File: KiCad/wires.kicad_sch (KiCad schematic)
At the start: 3 parts, among them U1 LT1762

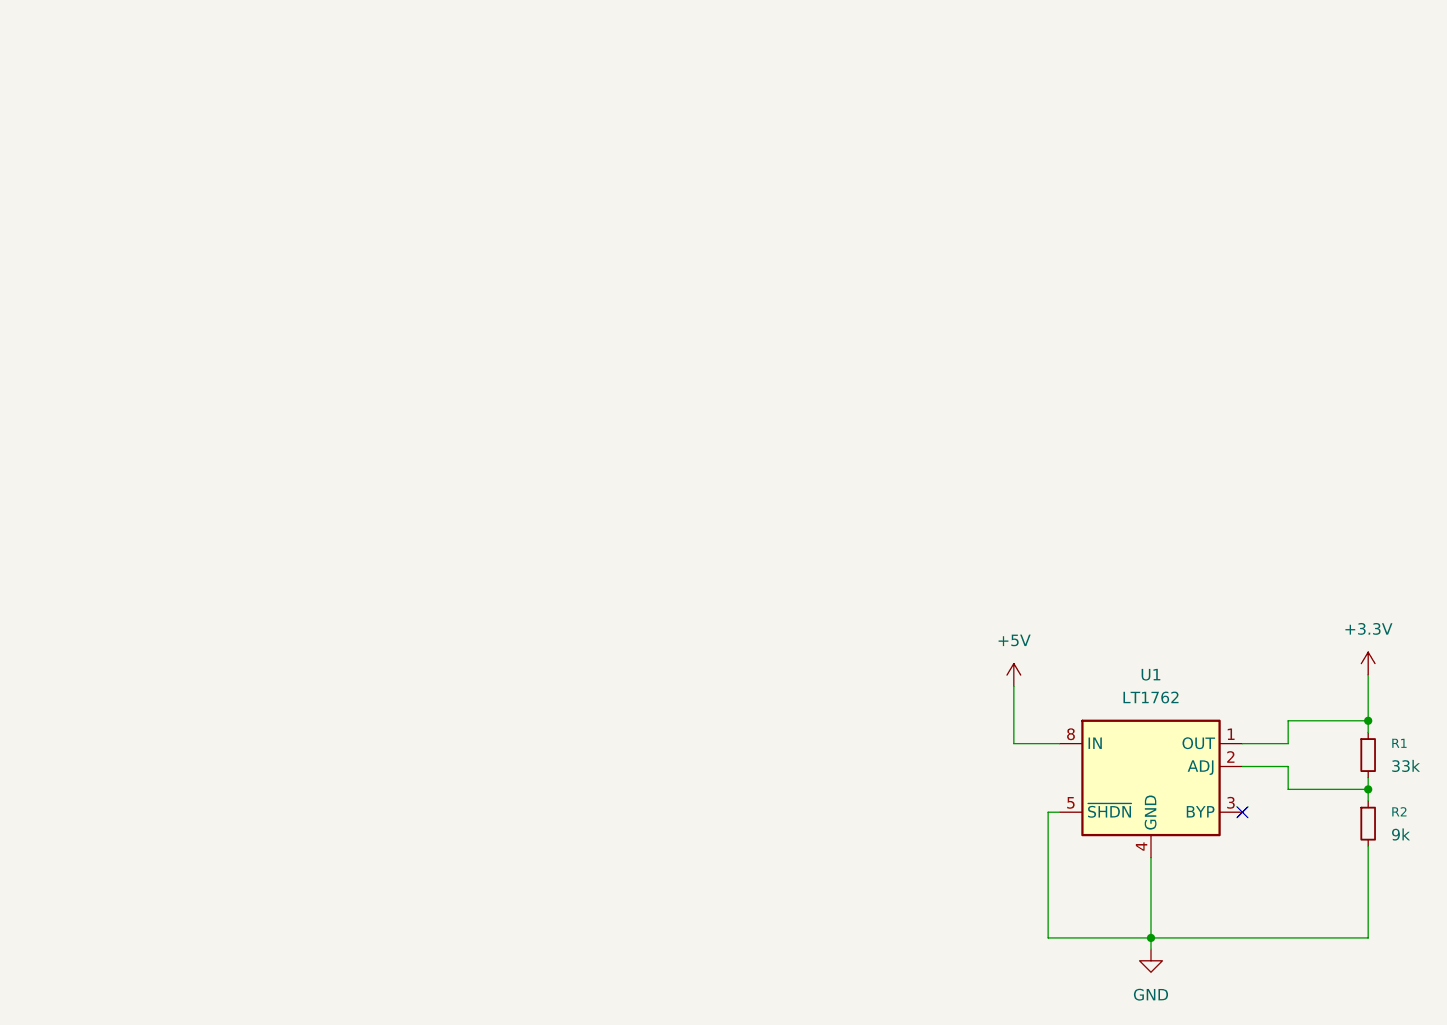
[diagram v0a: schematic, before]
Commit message: Update
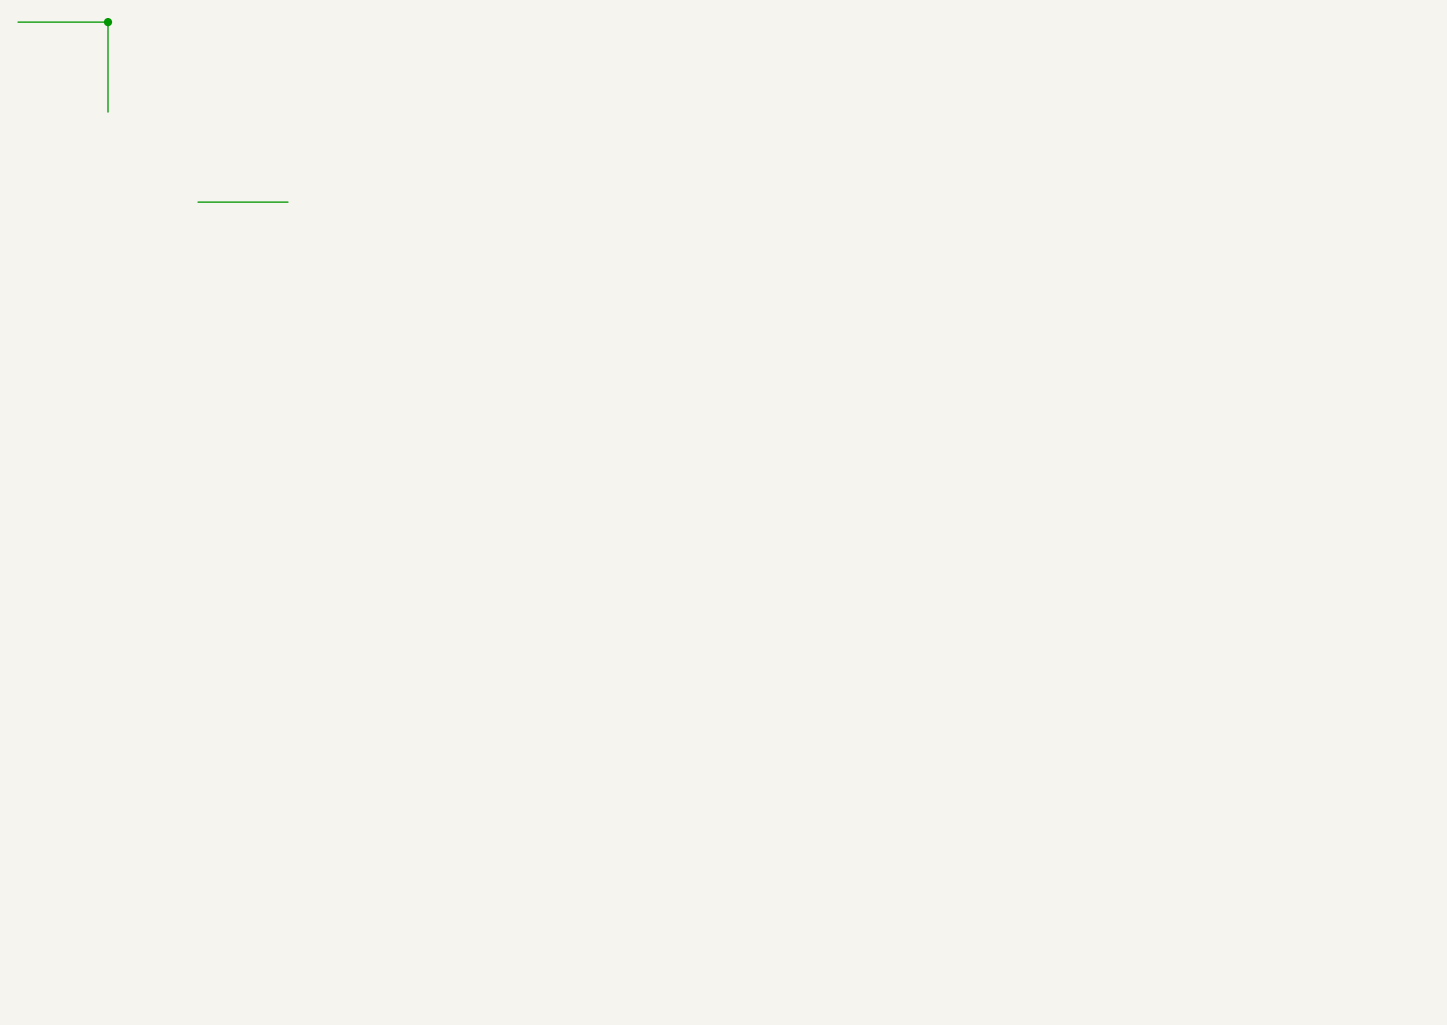
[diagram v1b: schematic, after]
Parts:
- removed R1: 33k, symbol Device:R_Small
- removed R2: 9k, symbol Device:R_Small
- removed U1: LT1762, Package_SO:MSOP-8_3x3mm_P0.65mm, symbol Regulator_Linear:LT1762
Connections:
- no-connect marks 1 -> 0
